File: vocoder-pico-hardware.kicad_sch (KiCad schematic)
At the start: 51 parts, among them J1 Conn_02x05_Odd_Even, J2 AudioJack2_SwitchT, J4 AudioJack2_SwitchT, SW1 SW_Push, SW2 SW_Push, U1 TL072, U2 LM7805_TO220, U3 PCM5100A, U8 MCP6002-xP, U9 TL072

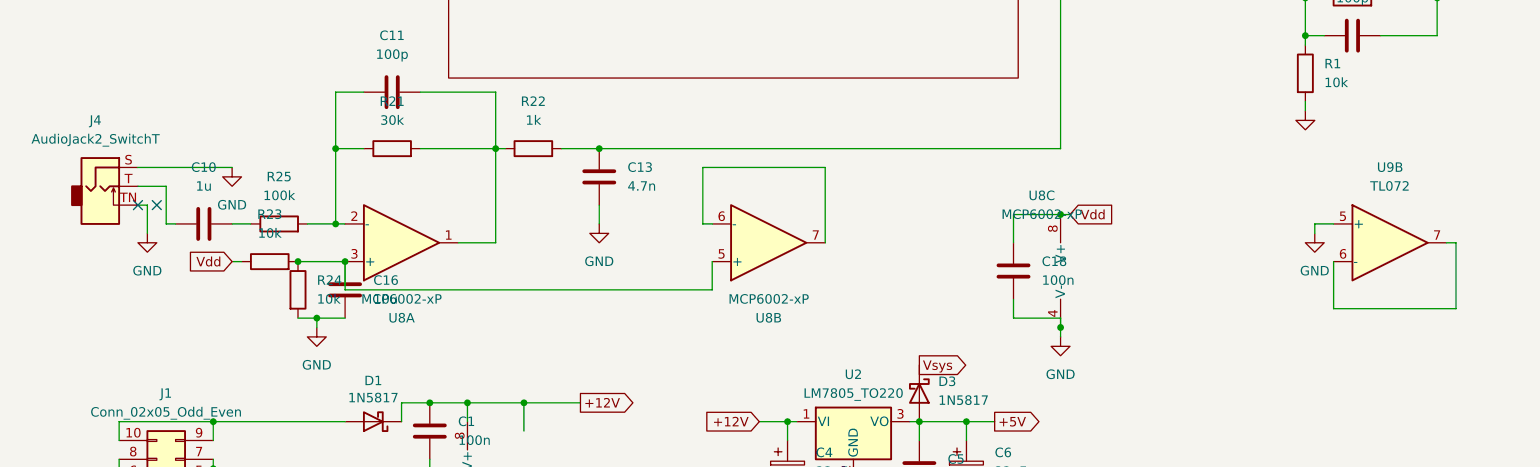
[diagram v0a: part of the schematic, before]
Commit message: final fixes
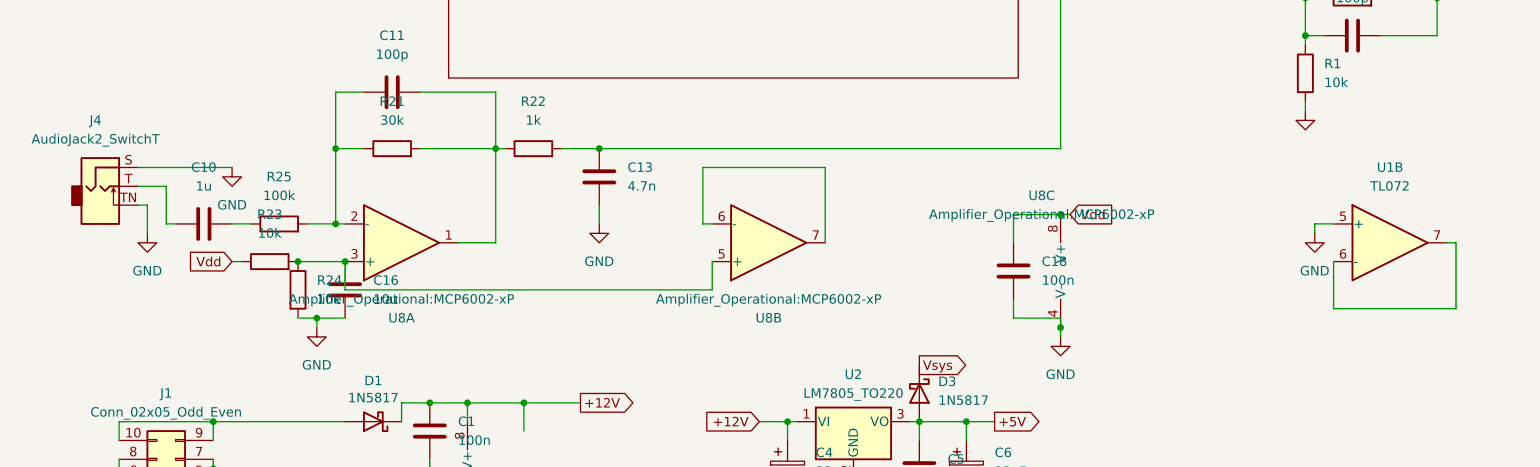
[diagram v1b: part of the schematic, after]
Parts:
- U8: value MCP6002-xP -> Amplifier_Operational:MCP6002-xP
- renumbered U9 to U1
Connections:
- no-connect marks 11 -> 9
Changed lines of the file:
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@@
 	)
 	(no_connect
-		(at 30.48 143.51)
-	)
-	(no_connect
 		(at 96.52 39.37)
 	)
 	(no_connect
-		(at 33.02 143.51)
-	)
-	(no_connect
 		(at 232.41 113.03)
 	)
@@
 	(wire
 		(pts
-			(xy 209.55 52.07) (xy 209.55 53.34)
+			(xy 30.48 143.51) (xy 31.75 143.51)
 		)
 		(stroke
@@
 	(wire
 		(pts
-			(xy 264.16 85.09) (xy 264.16 87.63)
+			(xy 209.55 52.07) (xy 209.55 53.34)
 		)
 		(stroke
@@
 	(wire
 		(pts
-			(xy 215.9 63.5) (xy 215.9 71.12)
+			(xy 264.16 85.09) (xy 264.16 87.63)
 		)
 		(stroke
@@
 	(wire
 		(pts
-			(xy 31.75 143.51) (xy 31.75 147.32)
+			(xy 215.9 63.5) (xy 215.9 71.12)
 		)
 		(stroke
@@
 	(wire
 		(pts
-			(xy 31.75 143.51) (xy 30.48 143.51)
-		)
-		(stroke
-			(width 0)
-			(type default)
-		)
-	)
-	(wire
-		(pts
 			(xy 247.65 63.5) (xy 250.19 63.5)
 		)
@@
 	(wire
 		(pts
+			(xy 31.75 143.51) (xy 31.75 147.32)
+		)
+		(stroke
+			(width 0)
+			(type default)
+		)
+	)
+	(wire
+		(pts
 			(xy 208.28 148.59) (xy 207.01 148.59)
 		)
@@
 			)
 		)
-		(property "Value" "MCP6002-xP"
+		(property "Value" "Amplifier_Operational:MCP6002-xP"
 			(at 66.04 156.21 0)
 			(effects
@@
 			)
 		)
-		(property "Value" "MCP6002-xP"
+		(property "Value" "Amplifier_Operational:MCP6002-xP"
 			(at 115.57 156.21 0)
 			(effects
@@
 		(dnp no)
 		(fields_autoplaced yes)
-		(property "Reference" "U9"
+		(property "Reference" "U1"
 			(at 199.39 138.43 0)
 			(effects
@@
 			(project "vocoder-pico-hardware"
 				(path "/68f2073a-7618-4fa5-a11d-b71bb4f75794"
-					(reference "U9")
+					(reference "U1")
 					(unit 2)
 				)
@@
 			)
 		)
-		(property "Value" "MCP6002-xP"
+		(property "Value" "Amplifier_Operational:MCP6002-xP"
 			(at 152.4 144.78 0)
 			(effects
